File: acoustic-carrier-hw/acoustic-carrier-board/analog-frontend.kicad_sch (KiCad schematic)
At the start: 88 parts, among them J1 BWU.FL-IPEX1, J10 BWU.FL-IPEX1, J11 BWU.FL-IPEX1, J17 BWU.FL-IPEX1, J22 8P8C_Shielded, J4 BWU.FL-IPEX1, J5 BWU.FL-IPEX1, J7 BWU.FL-IPEX1, U2 DGQ2788AEN-T1-GE4, U20 THS4521IDGK, U22 LMV321, U23 TL432DBZ, U3 MS9280

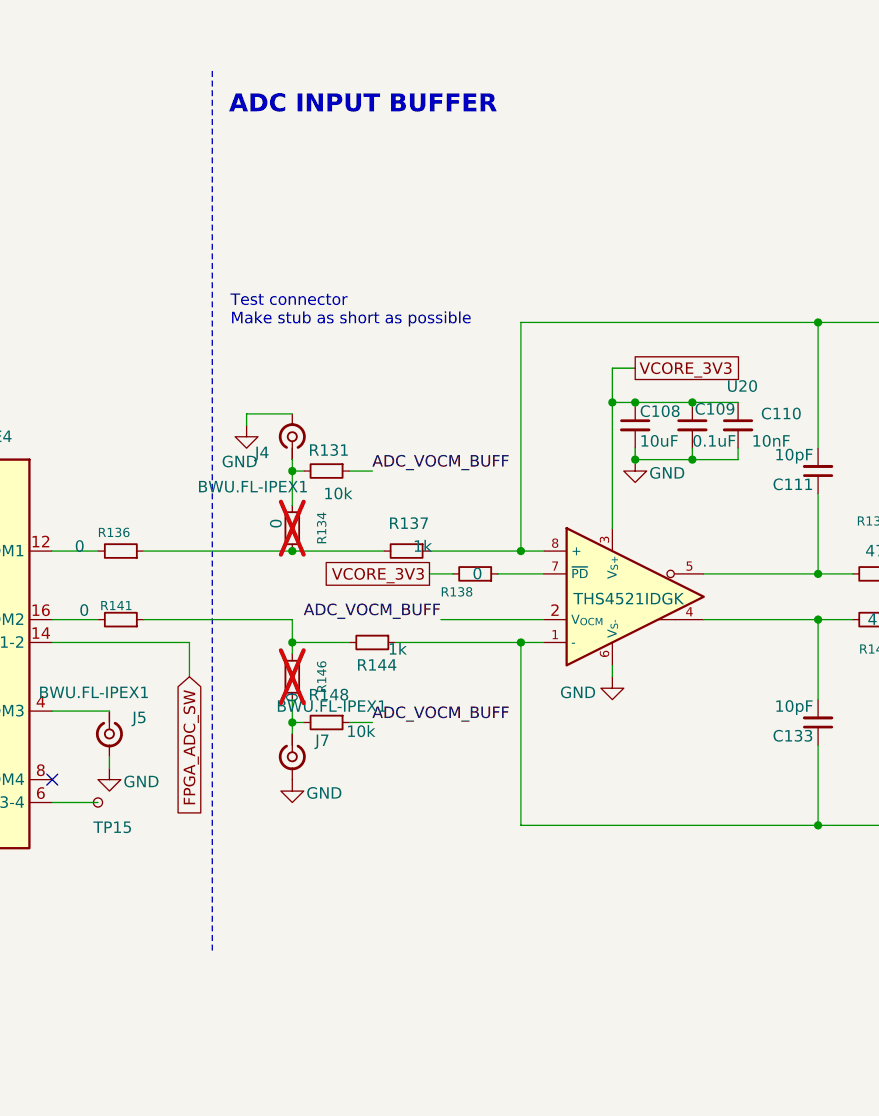
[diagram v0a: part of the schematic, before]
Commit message: [carrier] Did some check for example schematics, starting layout
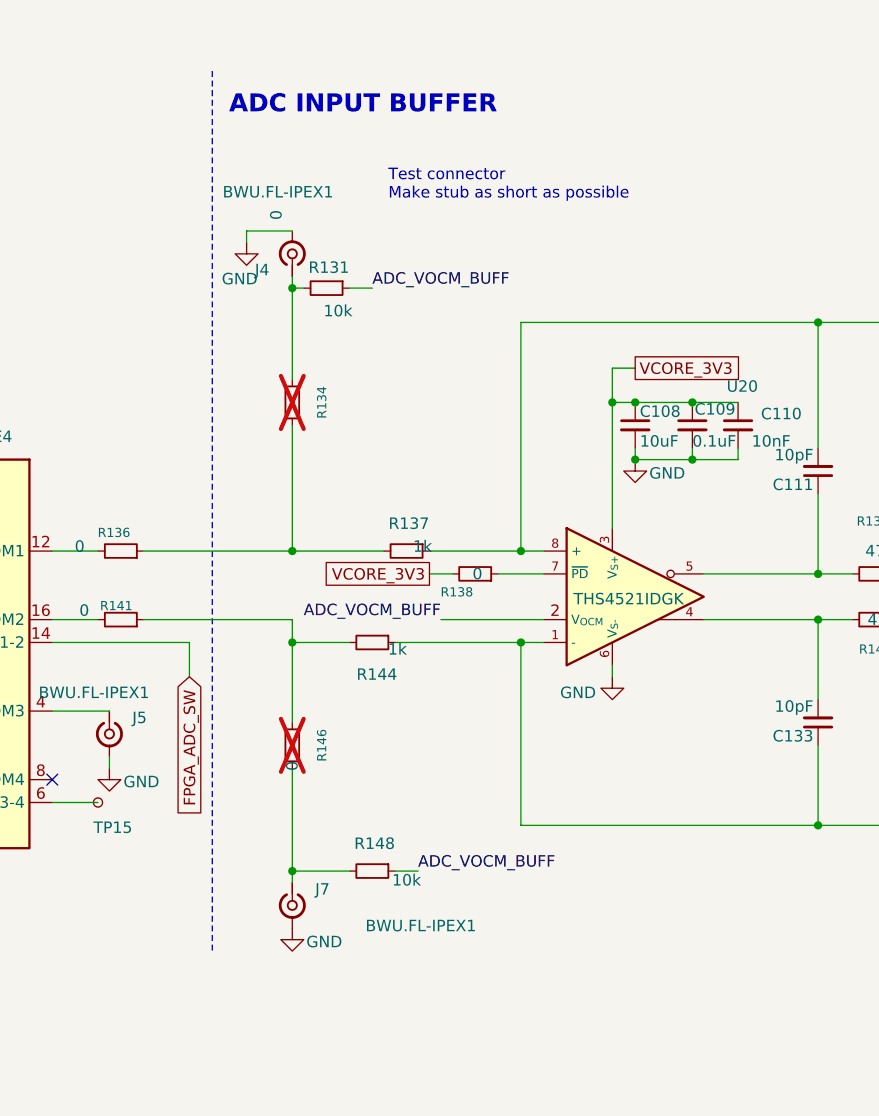
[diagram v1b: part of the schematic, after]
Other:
- moved on the sheet: J4, J7, R131, R134, R146, R148
